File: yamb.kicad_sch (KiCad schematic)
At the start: 5 parts, among them J1 Barrel_Jack, P1 USB_C_Plug_USB2.0

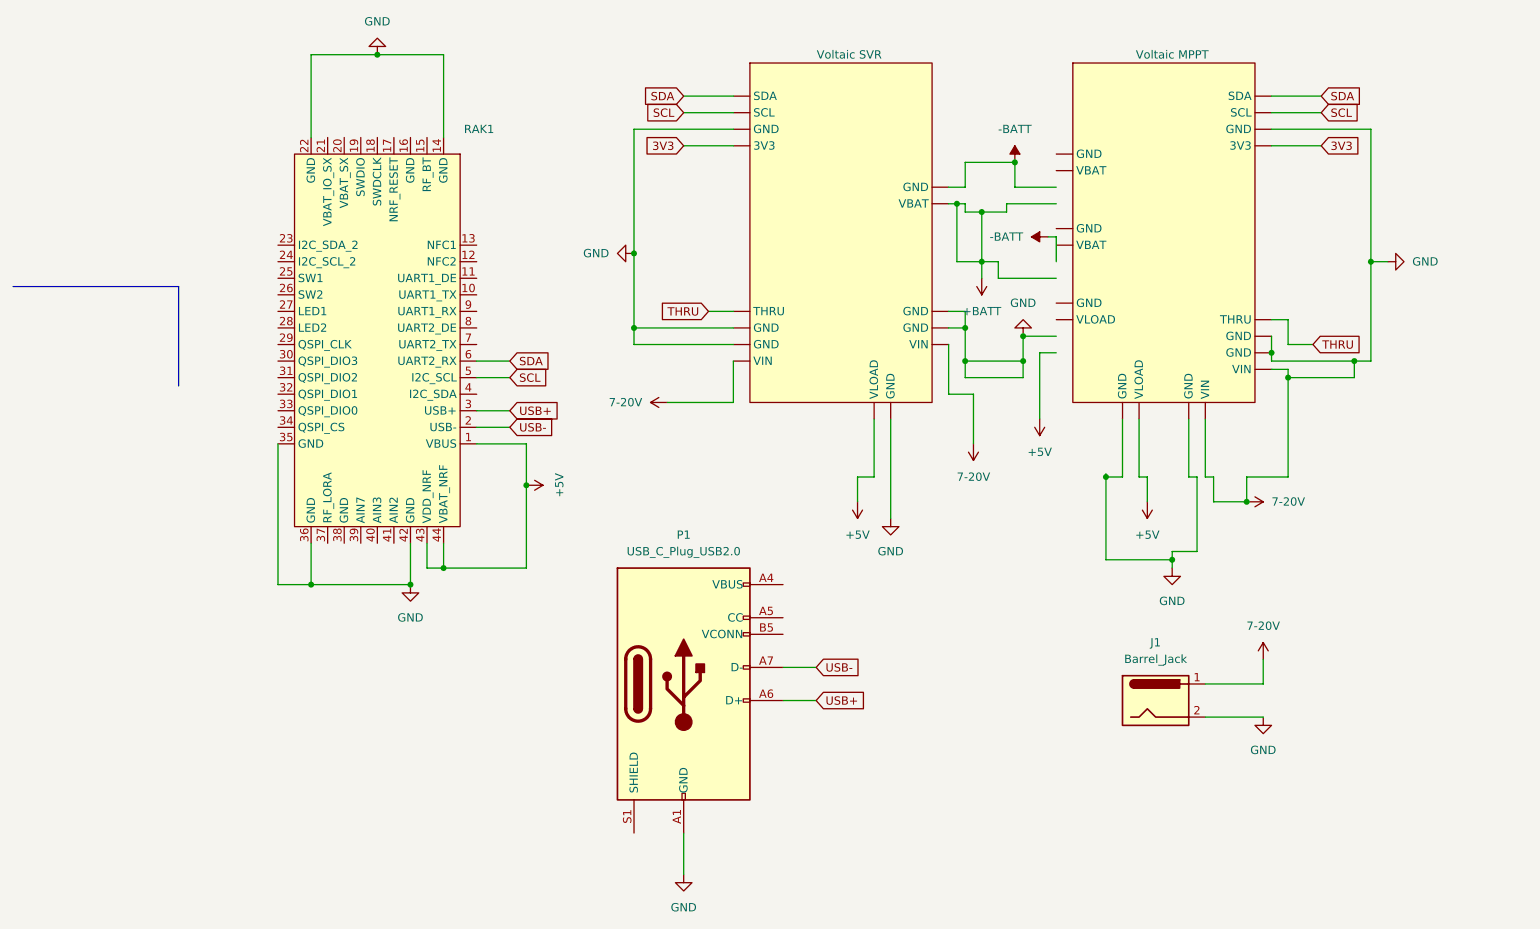
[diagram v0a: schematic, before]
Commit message: still lots of errors
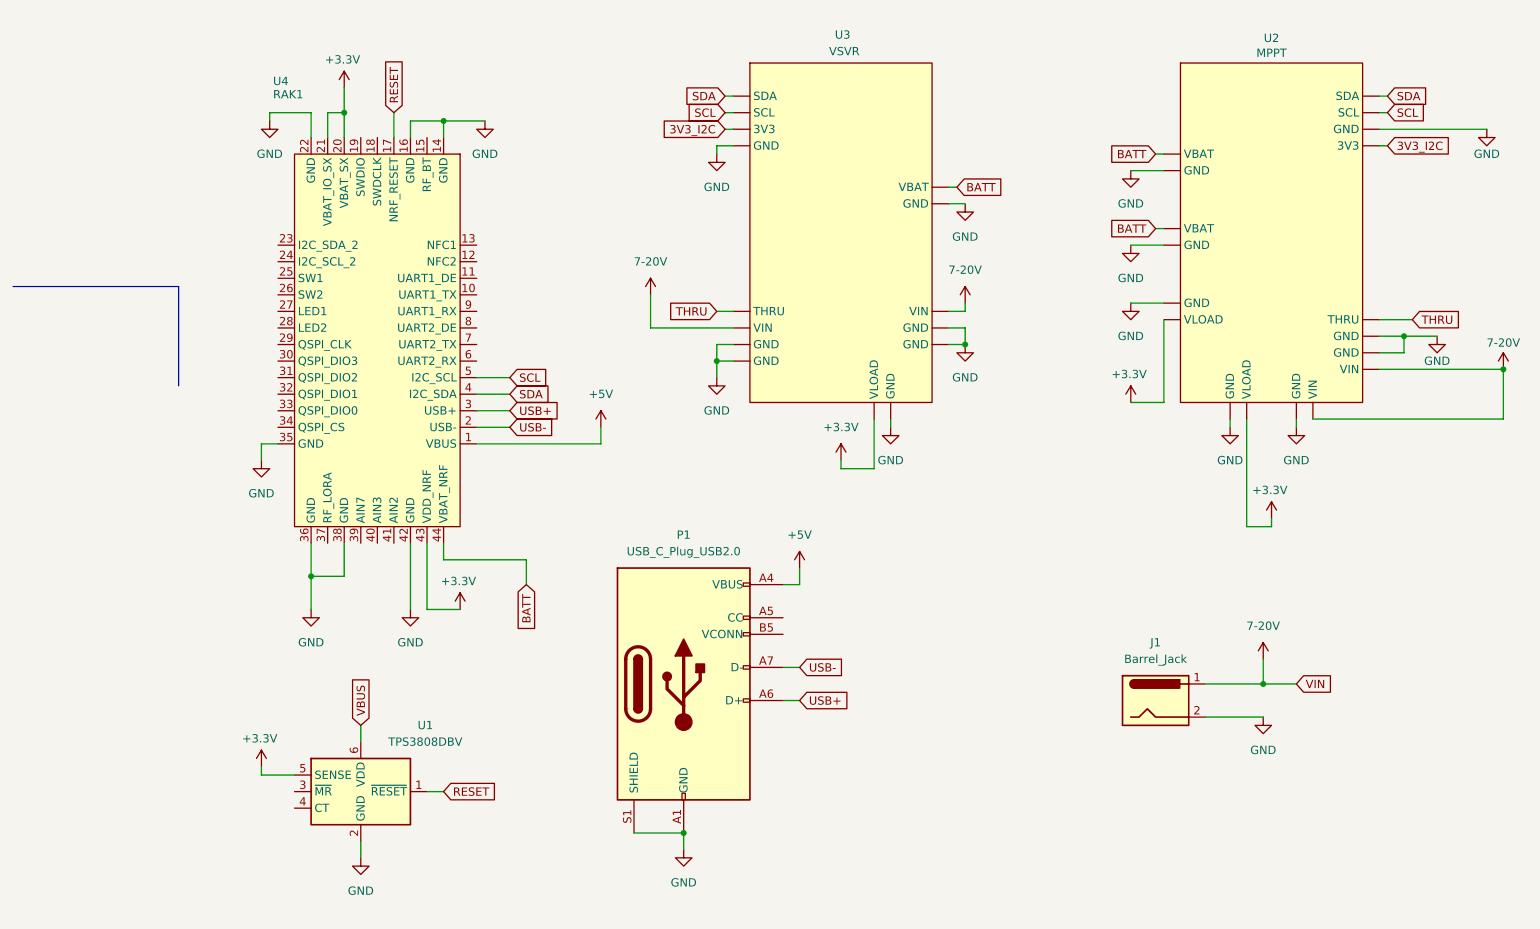
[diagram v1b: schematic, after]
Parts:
- added U1: TPS3808DBV, Package_TO_SOT_SMD:SOT-23-6, symbol Power_Supervisor:TPS3808DBV
- RAK1: value ~ -> U4
- U2: renamed from Voltaic MPPT; value ~ -> MPPT
- U3: renamed from Voltaic SVR; value ~ -> VSVR
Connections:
- net +BATT is gone; now on net BATT: U3.5 (VBAT)
- net -BATT is gone; now on net GND: U3.4 (GND)
- net +5V: now also P1.A4 (VBUS), P1.A9 (VBUS), P1.B4 (VBUS), P1.B9 (VBUS); no longer RAK1.43 (VDD_NRF), RAK1.44 (VBAT_NRF), U2.11 (VLOAD), U3.12 (VLOAD)
- net 7-20V: no longer J1.2, P1.A1 (GND), P1.A12 (GND), P1.B1 (GND), P1.B12 (GND), RAK1.14 (GND), RAK1.22 (GND), RAK1.35 (GND), RAK1.36 (GND), RAK1.42 (GND), U2.10 (GND), U2.12 (GND), U2.14 (GND), U2.16 (GND), U2.17 (GND), U3.13 (GND), U3.14 (GND), U3.16 (GND), U3.17 (GND), U3.7 (GND), U3.8 (GND)
- net SDA: now also RAK1.4 (I2C_SDA); no longer RAK1.6 (UART2_RX)
- net GND: now reaches P1.S1 (SHIELD)
- net GND: now also J1.2, P1.A1 (GND), P1.A12 (GND), P1.B1 (GND), P1.B12 (GND), RAK1.14 (GND), RAK1.16 (GND), RAK1.22 (GND), RAK1.35 (GND), RAK1.36 (GND), RAK1.38 (GND), RAK1.42 (GND), U2.10 (GND), U2.12 (GND), U2.14 (GND), U2.16 (GND), U2.17 (GND), U2.4 (GND), U2.6 (GND), U2.8 (GND), U3.13 (GND), U3.14 (GND), U3.16 (GND), U3.17 (GND), U3.7 (GND), U3.8 (GND), U1.2 (GND)
- net RESET: now reaches RAK1.17 (NRF_RESET)
- net RESET: now also U1.1 (~{RESET})
- net +3.3V: now reaches RAK1.20 (VBAT_SX)
- net +3.3V: now also RAK1.21 (VBAT_IO_SX), RAK1.43 (VDD_NRF), U2.11 (VLOAD), U2.9 (VLOAD), U3.12 (VLOAD), U1.5 (SENSE)
- net BATT: now reaches U2.5 (VBAT)
- net BATT: now also RAK1.44 (VBAT_NRF), U2.7 (VBAT)
- net 3V3 renamed 3V3_I2C
- new net VBUS: U1.6 (VDD)
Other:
- moved on the sheet: U2
